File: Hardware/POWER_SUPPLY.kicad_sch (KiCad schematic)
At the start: 57 parts, among them U10 REF3030AIDBZR, U4 LM5164DDAR, U5 MP1605GTF-Z, U61 RS621PXF, U7 JW5026, U8 MP1605GTF-Z, U9 LP5907MFX-3.3/NOPB

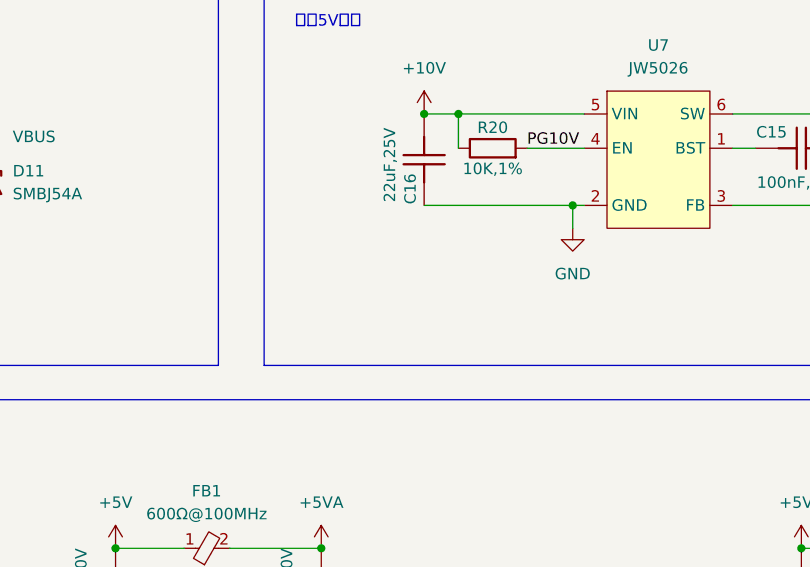
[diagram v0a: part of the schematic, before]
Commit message: 更改网口接地，更改RC吸收封装
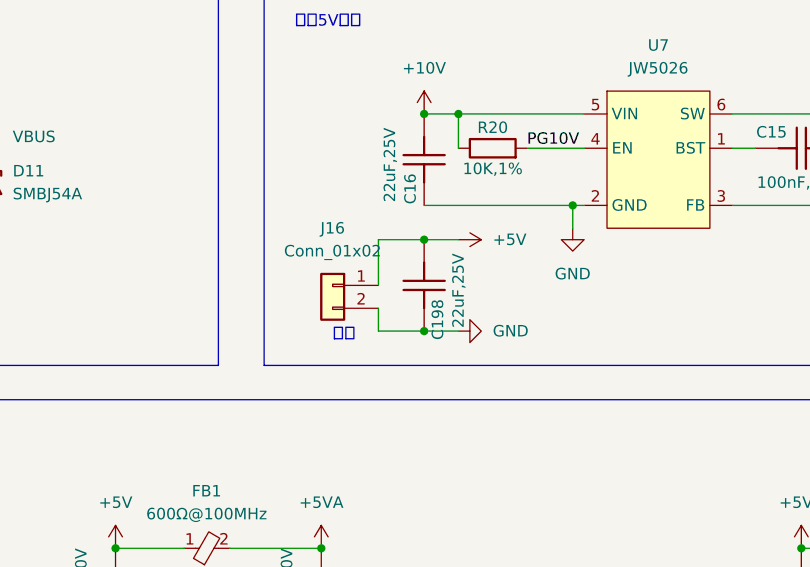
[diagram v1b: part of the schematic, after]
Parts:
- added C198: 22uF,25V, Capacitor_SMD:C_0805_2012Metric, symbol HPM6280Foc:CL21A226MAYNNNE
- added J16: Conn_01x02, Connector_JST:JST_PH_B2B-PH-K_1x02_P2.00mm_Vertical, symbol Connector_Generic:Conn_01x02
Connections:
- net +5V: now also C198.1, J16.1 (Pin_1)
- net GND: now also C198.2, J16.2 (Pin_2)
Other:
- note added: "风扇"

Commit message: PCB：风扇增加控制IO，泄放驱动增加使能引脚，485编码器电源接入控制
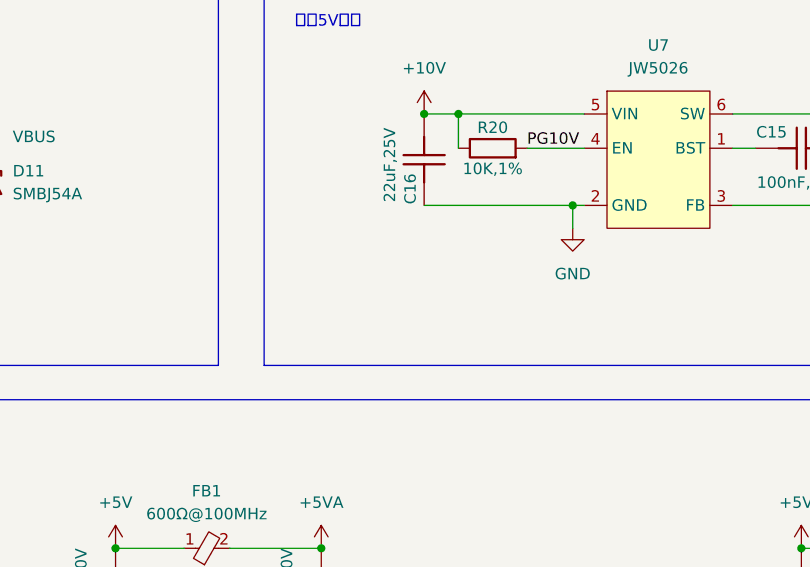
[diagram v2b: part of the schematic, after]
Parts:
- removed C198: 22uF,25V, Capacitor_SMD:C_0805_2012Metric, symbol HPM6280Foc:CL21A226MAYNNNE
- removed J16: Conn_01x02, Connector_JST:JST_PH_B2B-PH-K_1x02_P2.00mm_Vertical, symbol Connector_Generic:Conn_01x02
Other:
- note removed: "风扇"
